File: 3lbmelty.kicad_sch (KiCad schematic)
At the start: 20 parts, among them J1 Esc 2, J2 Amass_XT90-S, J3 Esc 1, Q1 SUM110P06-07L-E3, Q2 2N7002, U1 MCU, U2 Adafruit_H3LIS311_Breakout, U4 RC_RECEIVER, U5 BUCK_CONVERTER

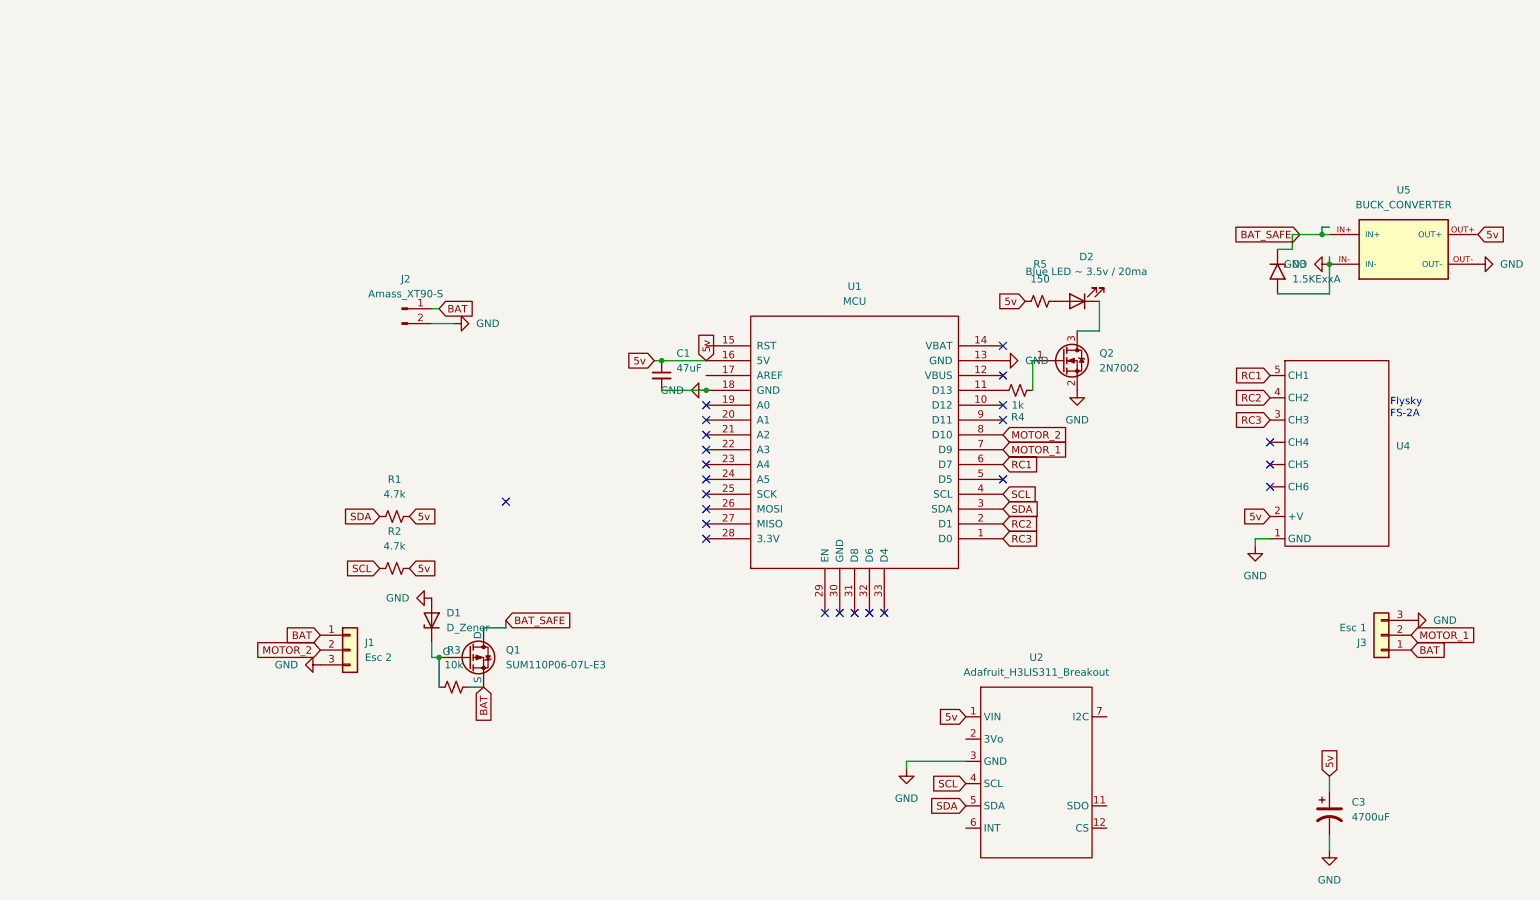
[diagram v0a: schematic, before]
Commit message: new pcb
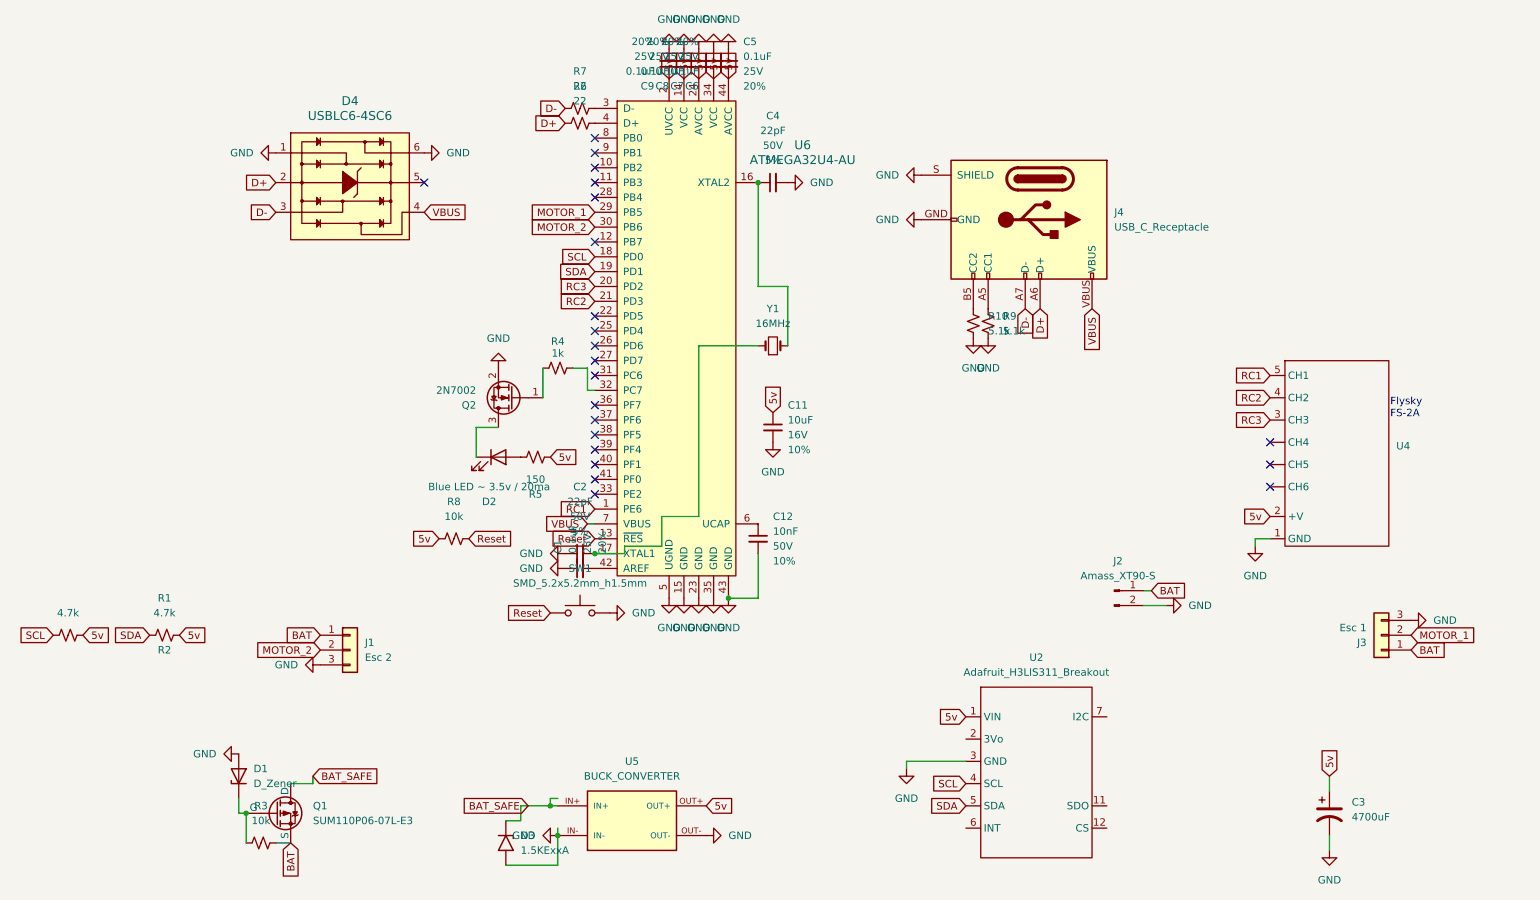
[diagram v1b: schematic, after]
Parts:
- removed C1: 47uF, SparkFun-Capacitor:C_0805_2012Metric, symbol SparkFun-Capacitor:47uF_0805_6.3V_20%
- removed U1: MCU, Adafruit-Eagle-Library.kicad:Adafruit ItsyBitsy 32u4 - 5V 16MHz, symbol Adafruit ItsyBitsy 32u4 - 5V 16MHz:MCU
- added C1, C5, C6, C7, C8, C9: 0.1uF, SparkFun-Capacitor:C_0603_1608Metric, symbol SparkFun-Capacitor:0.1uF_0603_25V_20%
- added C11: 10uF, SparkFun-Capacitor:C_0805_2012Metric, symbol SparkFun-Capacitor:10uF_0805_25V_10%
- added C12: 10nF, SparkFun-Capacitor:C_0603_1608Metric, symbol SparkFun-Capacitor:10nF_0603_50V_10%
- added C2, C4: 22pF, Capacitor_SMD:C_0603_1608Metric, symbol SparkFun-Capacitor:22pF_0402_50V_5%
- added D4: USBLC6-4SC6, digikey-footprints:SOT23-6L, symbol dk_TVS-Diodes:USBLC6-4SC6
- added J4: USB_C_Receptacle, SparkFun-Connector:USB-C_16, symbol SparkFun-Connector:USB_C_Receptacle
- added R10, R9: 5.1k, SparkFun-Resistor:R_0603_1608Metric, symbol SparkFun-Resistor:5.1k_0603
- added R6, R7: 22, SparkFun-Resistor:R_0603_1608Metric, symbol SparkFun-Resistor:22_0603
- added R8: 10k, SparkFun-Resistor:R_0603_1608Metric, symbol SparkFun-Resistor:10k_0603
- added SW1: SMD_5.2x5.2mm_h1.5mm, SparkFun-Switch:Push_SMD_5.2x5.2mm_h1.9mm, symbol SparkFun-Switch:SPST_Push_SMD_5.2x5.2mm_h1.9mm
- added U6: ATMEGA32U4-AU, digikey-footprints:TQFP-44_10x10mm, symbol dk_Embedded-Microcontrollers:ATMEGA32U4-AU
- added Y1: 16MHz, SparkFun-Clock:Crystal_SMD_2.0x1.6mm, symbol SparkFun-Clock:Crystal_16MHz_2.0x1.6mm
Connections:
- net 5v: now also C11.1, C5.2, C6.1, C7.1, C8.1, C9.1, R8.1, U6.14 (VCC), U6.2 (UVCC), U6.24 (AVCC), U6.34 (VCC), U6.44 (AVCC)
- net GND: now also C1.1, C11.2, C12.2, C2.1, C4.2, C5.1, C6.2, C7.2, C8.2, C9.2, D4.1, D4.6, J4.GND, J4.S (SHIELD), R10.1, R9.2, SW1.2, U6.15 (GND), U6.23 (GND), U6.35 (GND), U6.43 (GND), U6.5 (UGND)
- net MOTOR_1: now also U6.29 (PB5)
- net MOTOR_2: now also U6.30 (PB6)
- net RC1: now also U6.1 (PE6)
- net RC2: now also U6.21 (PD3)
- net RC3: now also U6.20 (PD2)
- net SCL: now also U6.18 (PD0)
- net SDA: now also U6.19 (PD1)
- net at R4.1: now also U6.32 (PC7)
- new net: C4.1, U6.16 (XTAL2), Y1.2
- new net: C2.2, U6.17 (XTAL1), Y1.1
- new net: R7.2, U6.3 (D-)
- new net: R6.2, U6.4 (D+)
- new net: C1.2, U6.42 (AREF)
- new net: C12.1, U6.6 (UCAP)
- new net: J4.A5 (CC1), R9.1
- new net: J4.B5 (CC2), R10.2
- new net D+: D4.2, J4.A6 (D+), J4.B6 (D+), R6.1
- new net D-: D4.3, J4.A7 (D-), J4.B7 (D-), R7.1
- new net Reset: R8.2, SW1.1, U6.13 (~{RES})
- new net VBUS: D4.4, J4.VBUS, U6.7 (VBUS)
- no-connect marks 24 -> 22
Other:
- moved on the sheet: D1, D2, D3, J2, Q1, Q2, R1, R2, R3, R4, R5, U5
